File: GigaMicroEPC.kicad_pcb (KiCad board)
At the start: 4 copper layers, 100 x 100 mm, 392 parts, among them J1 MAIN, J2 PRG CONN, Q1 EPC2304, Q10 EPC2304, Q11 EPC2304, Q12 EPC2304, Q13 EPC2304, Q14 EPC2304, Q15 EPC2304, Q16 EPC2304, Q17 EPC2304, Q18 EPC2304, Q19 EPC2304, Q2 EPC2304, Q20 EPC2304, Q21 EPC2304, Q3 EPC2304, Q4 EPC2304, Q5 EPC2304, Q6 EPC2304, Q7 CPC3980, Q8 IRFS4227TRLPBF, Q9 MMBTA92, U1 STM32F405RGT6, U10 STDRIVEG600, U11 ACS37030, U12 STDRIVEG600, U13 ACS37030, U14 STDRIVEG600, U15 ACS37030, U16 ESP32-C3-WROOM-02-N4, U2 LSM6DS3TR-C, U3 TJA1050T/CM,118, U4 TPS5430DDAR, U5 REF3033AIDBZR, U6 AMS1117-3.3, U7 TL494, U8 IR2181, U9 TL431, Y1 X50328MSB2GI

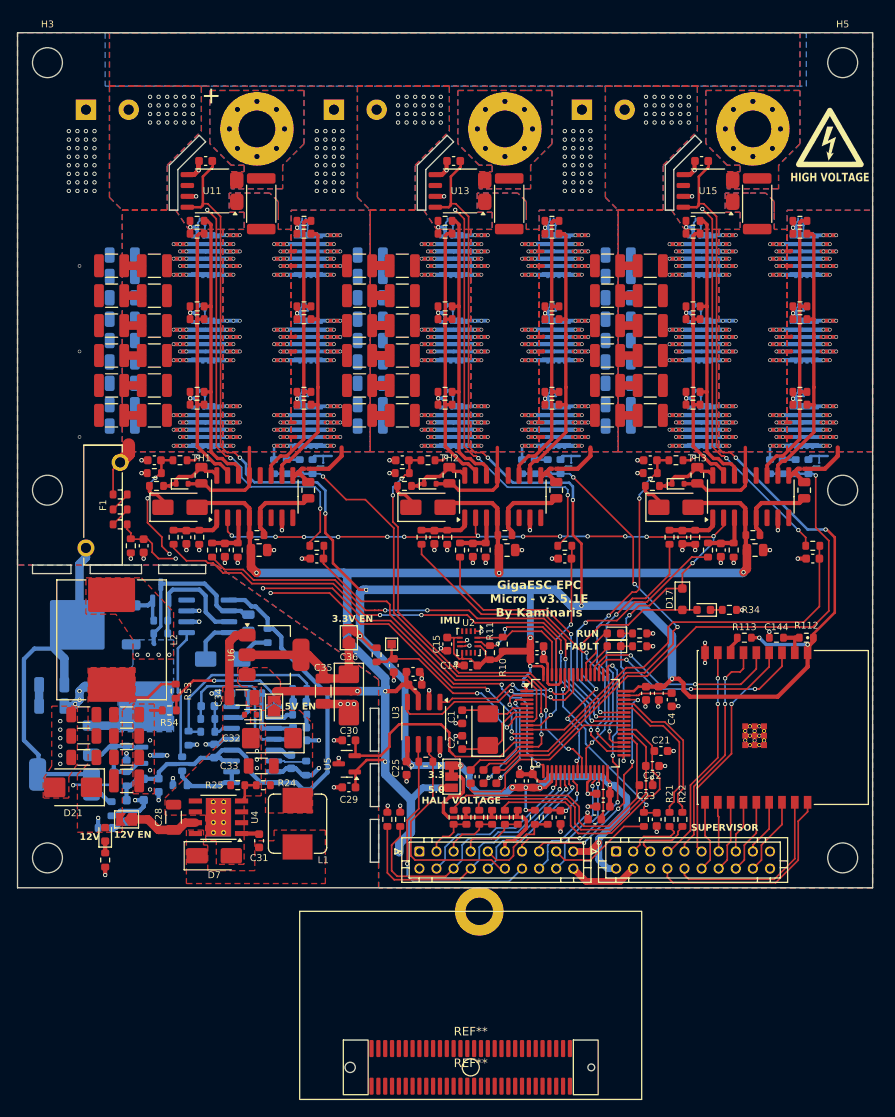
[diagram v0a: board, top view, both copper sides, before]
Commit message: modular
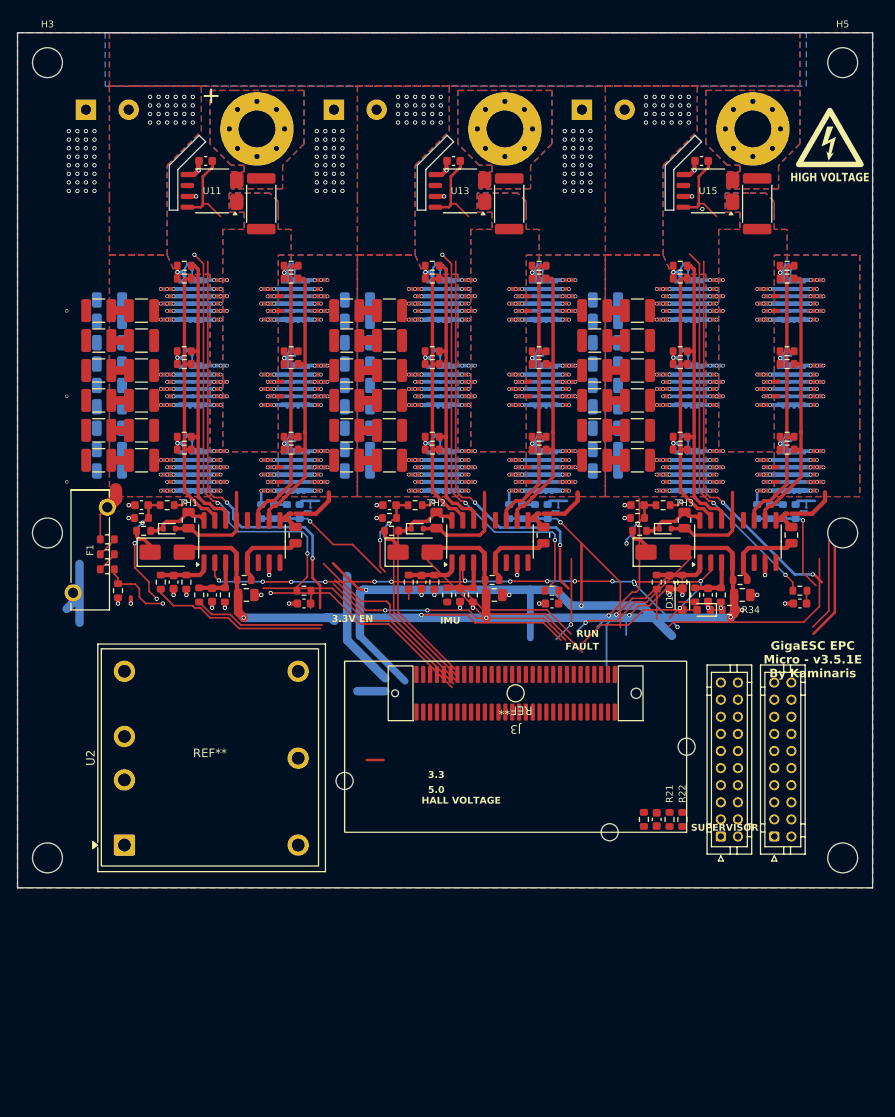
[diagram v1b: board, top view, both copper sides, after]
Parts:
- removed C1, C2: 20p, Capacitor_SMD:C_0603_1608Metric
- removed C10, C12, C13, C14, C15, C16, C17, C18, C24, C25, C37, C38, C40, C6, C8: 100n, Capacitor_SMD:C_0603_1608Metric
- removed C11, C31, C5, C7, C9: 10n, Capacitor_SMD:C_0603_1608Metric
- removed C144: 100n, GigaVescLibs:C_0603_1608Metric_L
- removed C19, C20, C21, C22, C23, C41, C43: 1n, Capacitor_SMD:C_0603_1608Metric
- removed C26: 2.2u, Capacitor_SMD:C_0603_1608Metric
- removed C28, C33, C34, C35, C48, C49, C50, C51, C52, C53: 22u, Capacitor_SMD:C_1206_3216Metric
- removed C29, C3, C30, C4, C42: 1u, Capacitor_SMD:C_0603_1608Metric
- removed C32, C36: 100uF 10V Tant, Capacitor_Tantalum_SMD:CP_EIA-6032-28_Kemet-C
- removed C39: 10u, Capacitor_SMD:C_0603_1608Metric
- removed C44: 100n 200V, Capacitor_SMD:C_0805_2012Metric
- removed C45, C46: 2.2u 100V, Capacitor_SMD:C_1206_3216Metric
- removed C47: 47u 16V, Capacitor_SMD:C_1210_3225Metric
- removed D1: L RUN, LED_SMD:LED_0603_1608Metric
- removed D18: BZT52C5V1S, Diode_SMD:D_SOD-323_HandSoldering
- removed D19: SS520F, Diode_SMD:D_SMA
- removed D2: L FAULT, LED_SMD:LED_0603_1608Metric
- removed D20: CI04S65E3, Package_TO_SOT_SMD:TO-252-2
- removed D21: BZG03C16-M3-08, Diode_SMD:D_SMB
- removed D22: 1N5819WS, Diode_SMD:D_SOD-323_HandSoldering
- removed D23: RUN, Diode_SMD:D_0603_1608Metric
- removed D57: MM5Z5V6ST1G, Diode_SMD:D_SOD-523
- removed D7: SS34, Diode_SMD:D_SMA
- removed JP1: VSel, Jumper:SolderJumper-3_P1.3mm_Bridged12_Pad1.0x1.5mm
- removed JP2: 5V-JMP, Jumper:SolderJumper-2_P1.3mm_Open_TrianglePad1.0x1.5mm
- removed JP3: 3.3V-JMP, Jumper:SolderJumper-2_P1.3mm_Open_TrianglePad1.0x1.5mm
- removed JP7: 12V-JMP, Jumper:SolderJumper-2_P1.3mm_Open_TrianglePad1.0x1.5mm
- removed L1: 15uH, Inductor_SMD:L_Bourns_SRP7028A_7.3x6.6mm
- removed L2: 100uH, Inductor_SMD:L_Chilisin_BMRG00131360
- removed Q7: CPC3980, Package_TO_SOT_SMD:SOT-223-3_TabPin2
- removed Q8: IRFS4227TRLPBF, Package_TO_SOT_SMD:TO-252-2
- removed Q9: MMBTA92, Package_TO_SOT_SMD:SOT-23
- removed R1, R112, R113, R12, R13, R14, R15, R16, R17, R18, R19, R2, R24, R3, R39, R4, R43, R44, R5, R50: 10k, Resistor_SMD:R_0603_1608Metric
- removed R10, R11, R40: 4.7k, Resistor_SMD:R_0603_1608Metric
- removed R20: 120, Resistor_SMD:R_0603_1608Metric
- removed R25: 3.3k, Resistor_SMD:R_0603_1608Metric
- removed R35: 200k, Resistor_SMD:R_0603_1608Metric
- removed R36, R37, R41: 5.1k, Resistor_SMD:R_0603_1608Metric
- removed R38: 2k, Resistor_SMD:R_0603_1608Metric
- removed R42, R45: 100, Resistor_SMD:R_0603_1608Metric
- removed R46, R51, R55: 22, Resistor_SMD:R_0603_1608Metric
- removed R47: 47, Resistor_SMD:R_0603_1608Metric
- removed R48: 30k, Resistor_SMD:R_0603_1608Metric
- removed R49: 9.1k, Resistor_SMD:R_0603_1608Metric
- removed R52: 1k, Resistor_SMD:R_0603_1608Metric
- removed R53: 100k, Resistor_SMD:R_0603_1608Metric
- removed R54: 27k, Resistor_SMD:R_0603_1608Metric
- removed R56: 82k, Resistor_SMD:R_0603_1608Metric
- removed the REF** at (163.0, 178.0)
- removed TP1: NRST, TestPoint:TestPoint_Pad_1.0x1.0mm
- removed U1: STM32F405RGT6, Package_QFP:LQFP-64_10x10mm_P0.5mm
- removed U16: ESP32-C3-WROOM-02-N4, GigaVescLibs:MODULE_ESP32-C3-WROOM-02-H4
- removed U3: TJA1050T/CM,118, Package_SO:SOIC-8_3.9x4.9mm_P1.27mm
- removed U4: TPS5430DDAR, Package_SO:TI_SO-PowerPAD-8_ThermalVias
- removed U5: REF3033AIDBZR, Package_TO_SOT_SMD:SOT-23
- removed U6: AMS1117-3.3, Package_TO_SOT_SMD:SOT-223-3_TabPin2
- removed U7: TL494, Package_SO:SOIC-16_3.9x9.9mm_P1.27mm
- removed U8: IR2181, Package_SO:SOIC-8_3.9x4.9mm_P1.27mm
- removed U9: TL431, Package_TO_SOT_SMD:SOT-23
- removed Y1: X50328MSB2GI, Crystal:Crystal_SMD_5032-2Pin_5.0x3.2mm
- added J3: Main Connector, GigaVescLibs:X0802FVS-60AS-LPV01, F.Cu at (168.2, 134.2)
- added REF**: TL494Brick, GigaVescLibs:TL494Brick, F.Cu at (132.5, 141.8)
- U2: value LSM6DS3TR-C -> THN10-7211UIR; footprint Package_LGA:Bosch_LGA-14_3x2.5mm_P0.5mm -> Converter_DCDC:Converter_DCDC_TRACO_THN10-xxxxUIR_THT
- moved U2 46.7 mm to (122.5, 152.0), turned to 90 degrees
- moved REF** 44.1 mm to (168.2, 134.2), turned to 180 degrees
- moved J1 35.3 mm to (192.2, 151.0), turned to 90 degrees
- moved J2 18.6 mm to (198.5, 151.0), turned to 90 degrees
- moved C100 5.46 mm to (148.5, 96.5)
- moved C102 5.46 mm to (153.5, 93.0)
- moved C103 5.46 mm to (148.5, 93.0)
- moved C104 5.46 mm to (153.5, 100.0)
- moved C105 5.46 mm to (148.5, 100.0)
- moved C106 5.46 mm to (172.5, 123.8)
- moved C107 5.46 mm to (153.5, 89.5)
- moved C108 5.46 mm to (148.5, 89.5)
- moved C110 5.46 mm to (153.5, 103.5)
- moved C111 5.46 mm to (148.5, 103.5)
- moved C112 5.46 mm to (153.5, 107.0)
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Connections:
- J1 pad 6: ADC EXT -> SPI1 SCK
- J1 pad 8: ADC EXT2 -> SPI1 MISO
- U2 pad 1: GND -> unconnected-(U2-BUS-Pad1)
- U2 pad 2: unconnected-(U2-ASDx-Pad2) -> +VSW
- U2 pad 3: unconnected-(U2-ASCx-Pad3) -> GND
- U2 pad 4: unconnected-(U2-INT1-Pad4) -> Net-(SW1-B)
- U2 pad 5: +3.3V -> +12V
- U2 pad 6: GND -> unconnected-(U2-Trim-Pad6)
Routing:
- net +3.3V: track 420.7 -> 287.7 mm, vias 26 -> 11
- net +5V: track 201.0 -> 120.2 mm, vias 8 -> 3
- net GND: track 546.6 -> 473.7 mm, vias 317 -> 249
- net STARTUP: track 59.5 -> 0.00 mm
- net VSENSE3: track 67.3 -> 12.4 mm
- net L1: track 67.3 -> 26.0 mm, vias 4 -> 0
- net L2: track 39.6 -> 1.17 mm, vias 2 -> 0
- net HALL1: track 34.4 -> 0.00 mm
- net ADC EXT2: track 34.0 -> 0.00 mm, vias 1 -> 0
- net HALL2: track 33.7 -> 0.00 mm
- net HALL3: track 33.3 -> 0.00 mm
- net ADC EXT: track 32.8 -> 0.00 mm, vias 1 -> 0
- net H2: track 32.8 -> 0.00 mm, vias 2 -> 0
- net SWCLK: track 32.2 -> 0.00 mm, vias 4 -> 0
- net VSENSE2: track 58.0 -> 27.5 mm
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- removed copper zone on B.Cu, net (none)
- removed copper zone on F.Cu, net (none)
- removed copper zone on F.Cu, net +12V
- removed copper zone on F.Cu, net +5V
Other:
- outline, holes or cut-outs redrawn
- board text removed: "12V"
- board text removed: "12V EN"
- board text removed: "5V EN"
